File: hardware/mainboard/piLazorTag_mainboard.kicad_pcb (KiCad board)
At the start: 2 copper layers, 83.8 x 58.2 mm, 11 parts, among them M1 LOGIC_LEVEL_CONVERTER

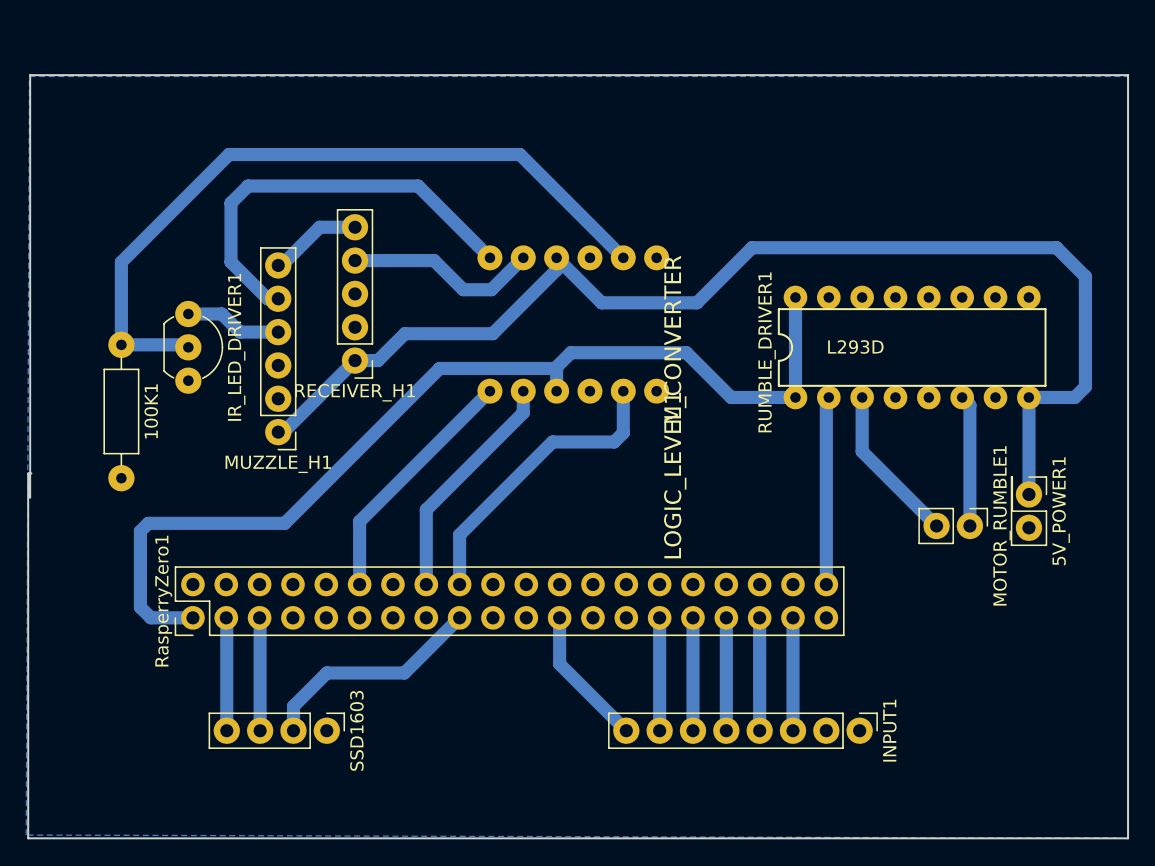
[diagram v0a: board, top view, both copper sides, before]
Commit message: Some new sender gerber stuff
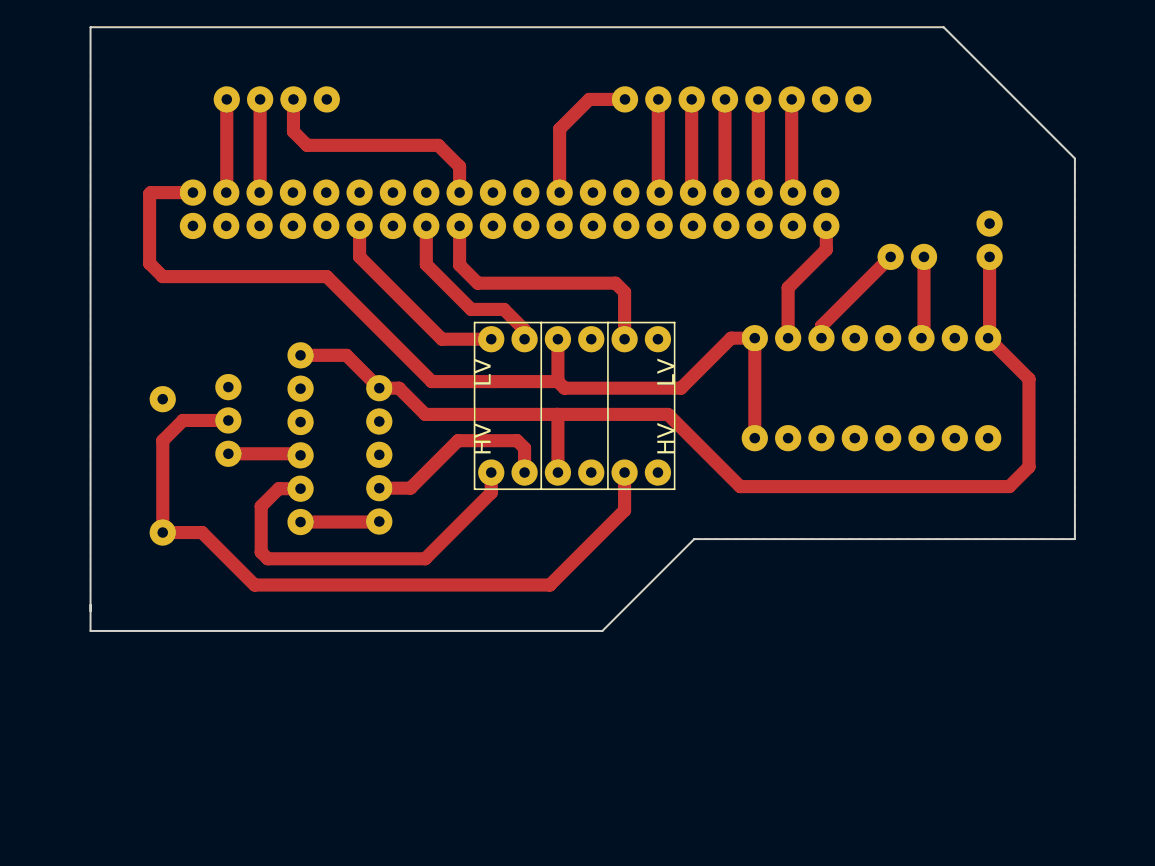
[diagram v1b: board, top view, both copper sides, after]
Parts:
- 100K1, 5V_POWER1, INPUT1, IR_LED_DRIVER1, M1, MOTOR_RUMBLE1, MUZZLE_H1, RECEIVER_H1, RUMBLE_DRIVER1, RasperryZero1, SSD1603: moved to B.Cu
- moved INPUT1 48.1 mm to (150.5, 73.5), turned to 90 degrees
- moved SSD1603 48.1 mm to (110.0, 73.5), turned to 90 degrees
- moved RasperryZero1 32.4 mm to (99.8, 80.6), turned to 270 degrees
- moved MOTOR_RUMBLE1 20.8 mm to (155.5, 85.5), turned to 90 degrees
- moved 5V_POWER1 18.3 mm to (160.5, 85.5), turned to 90 degrees
- moved 100K1 14.6 mm to (97.5, 106.5), turned to 90 degrees
- moved IR_LED_DRIVER1 11.1 mm to (102.5, 100.5), turned to 90 degrees
- moved M1 6.50 mm to (136.5, 90.5), turned to 270 degrees
- moved MUZZLE_H1 6.09 mm to (108.0, 93.0)
- moved RUMBLE_DRIVER1 4.38 mm to (151.5, 95.5)
- moved RECEIVER_H1 2.80 mm to (114.0, 95.5)
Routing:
- net +5V: track 93.5 -> 82.3 mm
- net /G23: track 17.8 -> 13.2 mm
- net /G21: track 14.3 -> 9.76 mm
- net +3V3: track 93.8 -> 89.3 mm
- net /G18: track 19.1 -> 15.2 mm
- net Net-(MOTOR_RUMBLE1-Pad2): track 12.1 -> 8.37 mm
- net Net-(MOTOR_RUMBLE1-Pad1): track 10.0 -> 6.27 mm
- net /M_LED_DI: track 31.8 -> 28.4 mm
- net /G24: track 22.7 -> 20.0 mm
- net /LED_IR_GND: track 7.42 -> 5.55 mm
- net Net-(100K1-Pad1): track 56.4 -> 54.7 mm
- net /G13: track 8.88 -> 7.42 mm
- net /G6: track 8.60 -> 7.14 mm
- net /G19: track 8.60 -> 7.14 mm
- net /G5: track 8.88 -> 7.42 mm
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- added copper zone on F.Cu, net GND
- removed copper zone on B.Cu, net GND
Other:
- board size 83.8 x 58.2 mm -> 75 x 46 mm
